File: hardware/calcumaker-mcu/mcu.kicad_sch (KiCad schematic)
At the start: 20 parts, among them J3 TO DISPLAY (unified SPI FFC), J4 SWD TC2030-NL, J7 VSYS -> matrix LED pwr, U1 STM32U575RGT6, Y1 32.768kHz

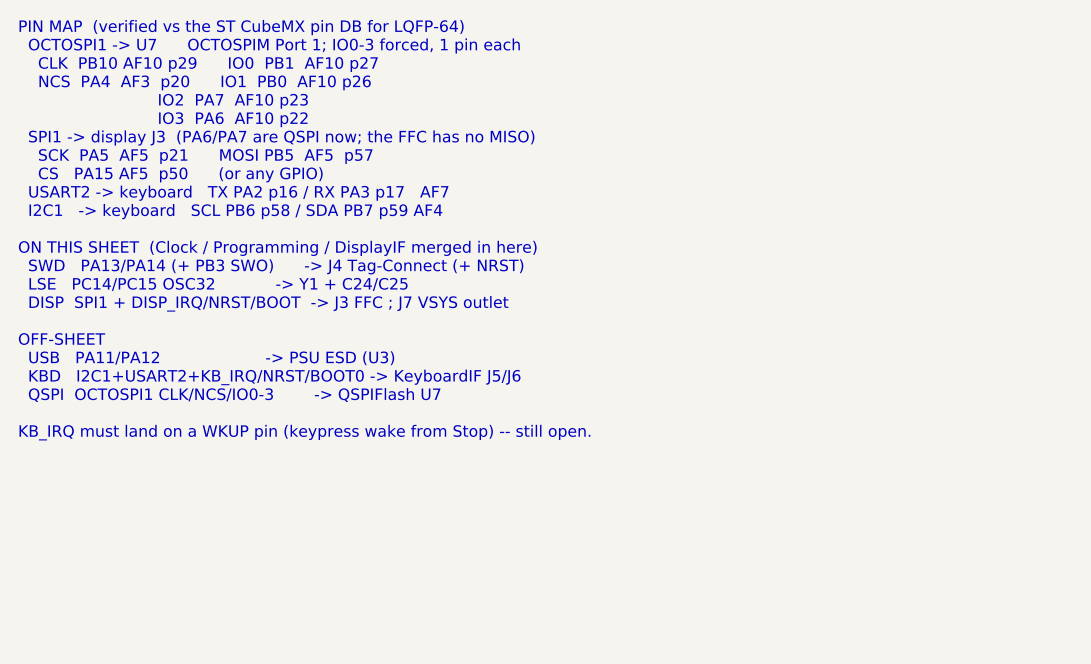
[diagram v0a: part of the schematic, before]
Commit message: Checkpoint
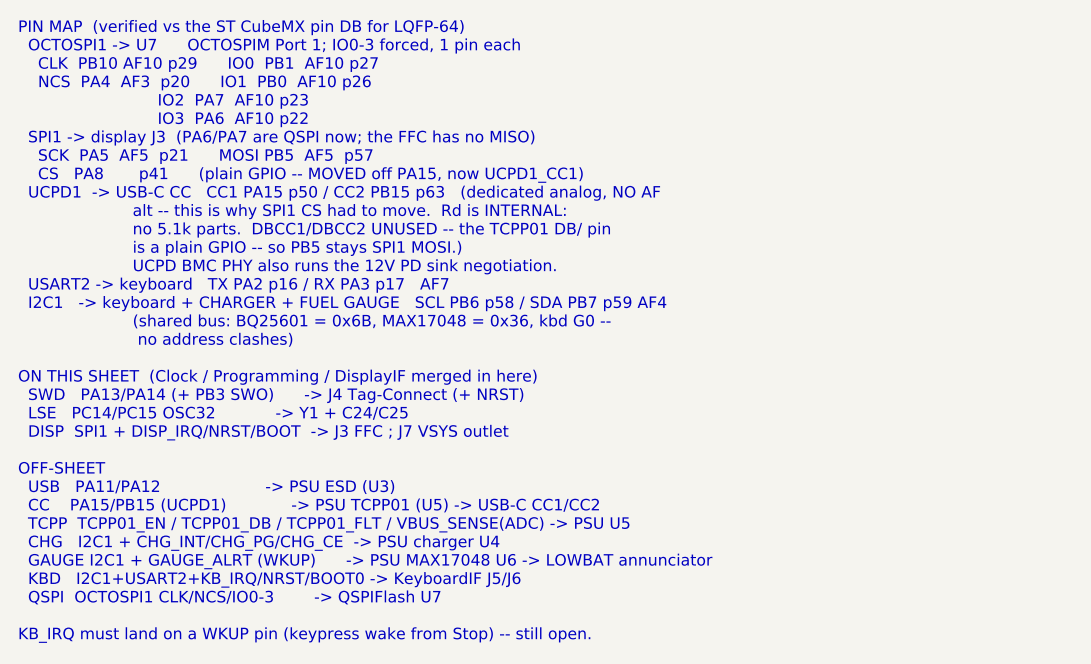
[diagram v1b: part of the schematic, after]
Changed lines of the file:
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@@
 		)
 	)
-	(text "MCU CORE  -  U1  STM32U575RGT6   (LQFP-64, Cortex-M33)\nSmaller pkg now the key matrix scans on the keyboard G0, not here.\n\nPOWER\n  VDD (each pin) -> +3V3   C12-C16 100nF + C17 10uF bulk\n                           (LQFP-64 has fewer VDD than the 5 caps;\n                            spares are extra bypass, trim @ layout)\n  VDDA / VREF+   -> +3V3   C18 1uF + C19 100nF\n  VDDUSB         -> +3V3   C20 100nF\n  VSS / EP       -> GND\n  VCORE          -> LDO or internal SMPS (SMPS: L on VLXSMPS + VDD12);\n                    C22/C23 = VCAP placeholders (set per mode)\nRESET / BOOT\n  NRST -> C21 100nF          BOOT0 -> R8 10k to GND\n\nPIN MAP  (verified vs the ST CubeMX pin DB for LQFP-64)\n  OCTOSPI1 -> U7      OCTOSPIM Port 1; IO0-3 forced, 1 pin each\n    CLK  PB10 AF10 p29      IO0  PB1  AF10 p27\n    NCS  PA4  AF3  p20      IO1  PB0  AF10 p26\n                            IO2  PA7  AF10 p23\n                            IO3  PA6  AF10 p22\n  SPI1 -> display J3  (PA6/PA7 are QSPI now; the FFC has no MISO)\n    SCK  PA5  AF5  p21      MOSI PB5  AF5  p57\n    CS   PA15 AF5  p50      (or any GPIO)\n  USART2 -> keyboard   TX PA2 p16 / RX PA3 p17   AF7\n  I2C1   -> keyboard   SCL PB6 p58 / SDA PB7 p59 AF4\n\nON THIS SHEET  (Clock / Programming / DisplayIF merged in here)\n  SWD   PA13/PA14 (+ PB3 SWO)      -> J4 Tag-Connect (+ NRST)\n  LSE   PC14/PC15 OSC32            -> Y1 + C24/C25\n  DISP  SPI1 + DISP_IRQ/NRST/BOOT  -> J3 FFC ; J7 VSYS outlet\n\nOFF-SHEET\n  USB   PA11/PA12                     -> PSU ESD (U3)\n  KBD   I2C1+USART2+KB_IRQ/NRST/BOOT0 -> KeyboardIF J5/J6\n  QSPI  OCTOSPI1 CLK/NCS/IO0-3        -> QSPIFlash U7\n\nKB_IRQ must land on a WKUP pin (keypress wake from Stop) -- still open."
+	(text "MCU CORE  -  U1  STM32U575RGT6   (LQFP-64, Cortex-M33)\nSmaller pkg now the key matrix scans on the keyboard G0, not here.\n\nPOWER\n  VDD (each pin) -> +3V3   C12-C16 100nF + C17 10uF bulk\n                           (LQFP-64 has fewer VDD than the 5 caps;\n                            spares are extra bypass, trim @ layout)\n  VDDA / VREF+   -> +3V3   C18 1uF + C19 100nF\n  VDDUSB         -> +3V3   C20 100nF\n  VSS / EP       -> GND\n  VCORE          -> LDO or internal SMPS (SMPS: L on VLXSMPS + VDD12);\n                    C22/C23 = VCAP placeholders (set per mode)\nRESET / BOOT\n  NRST -> C21 100nF          BOOT0 -> R8 10k to GND\n\nPIN MAP  (verified vs the ST CubeMX pin DB for LQFP-64)\n  OCTOSPI1 -> U7      OCTOSPIM Port 1; IO0-3 forced, 1 pin each\n    CLK  PB10 AF10 p29      IO0  PB1  AF10 p27\n    NCS  PA4  AF3  p20      IO1  PB0  AF10 p26\n                            IO2  PA7  AF10 p23\n                            IO3  PA6  AF10 p22\n  SPI1 -> display J3  (PA6/PA7 are QSPI now; the FFC has no MISO)\n    SCK  PA5  AF5  p21      MOSI PB5  AF5  p57\n    CS   PA8       p41      (plain GPIO -- MOVED off PA15, now UCPD1_CC1)\n  UCPD1  -> USB-C CC   CC1 PA15 p50 / CC2 PB15 p63   (dedicated analog, NO AF\n                       alt -- this is why SPI1 CS had to move.  Rd is INTERNAL:\n                       no 5.1k parts.  DBCC1/DBCC2 UNUSED -- the TCPP01 DB/ pin\n                       is a plain GPIO -- so PB5 stays SPI1 MOSI.)\n                       UCPD BMC PHY also runs the 12V PD sink negotiation.\n  USART2 -> keyboard   TX PA2 p16 / RX PA3 p17   AF7\n  I2C1   -> keyboard + CHARGER + FUEL GAUGE   SCL PB6 p58 / SDA PB7 p59 AF4\n                       (shared bus: BQ25601 = 0x6B, MAX17048 = 0x36, kbd G0 --\n                        no address clashes)\n\nON THIS SHEET  (Clock / Programming / DisplayIF merged in here)\n  SWD   PA13/PA14 (+ PB3 SWO)      -> J4 Tag-Connect (+ NRST)\n  LSE   PC14/PC15 OSC32            -> Y1 + C24/C25\n  DISP  SPI1 + DISP_IRQ/NRST/BOOT  -> J3 FFC ; J7 VSYS outlet\n\nOFF-SHEET\n  USB   PA11/PA12                     -> PSU ESD (U3)\n  CC    PA15/PB15 (UCPD1)             -> PSU TCPP01 (U5) -> USB-C CC1/CC2\n  TCPP  TCPP01_EN / TCPP01_DB / TCPP01_FLT / VBUS_SENSE(ADC) -> PSU U5\n  CHG   I2C1 + CHG_INT/CHG_PG/CHG_CE  -> PSU charger U4\n  GAUGE I2C1 + GAUGE_ALRT (WKUP)      -> PSU MAX17048 U6 -> LOWBAT annunciator\n  KBD   I2C1+USART2+KB_IRQ/NRST/BOOT0 -> KeyboardIF J5/J6\n  QSPI  OCTOSPI1 CLK/NCS/IO0-3        -> QSPIFlash U7\n\nKB_IRQ must land on a WKUP pin (keypress wake from Stop) -- still open."
 		(exclude_from_sim no)
 		(at 15 168.4 0)
